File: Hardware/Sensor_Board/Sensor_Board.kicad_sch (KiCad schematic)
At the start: 3 parts, among them J2 Conn_02x20_Odd_Even

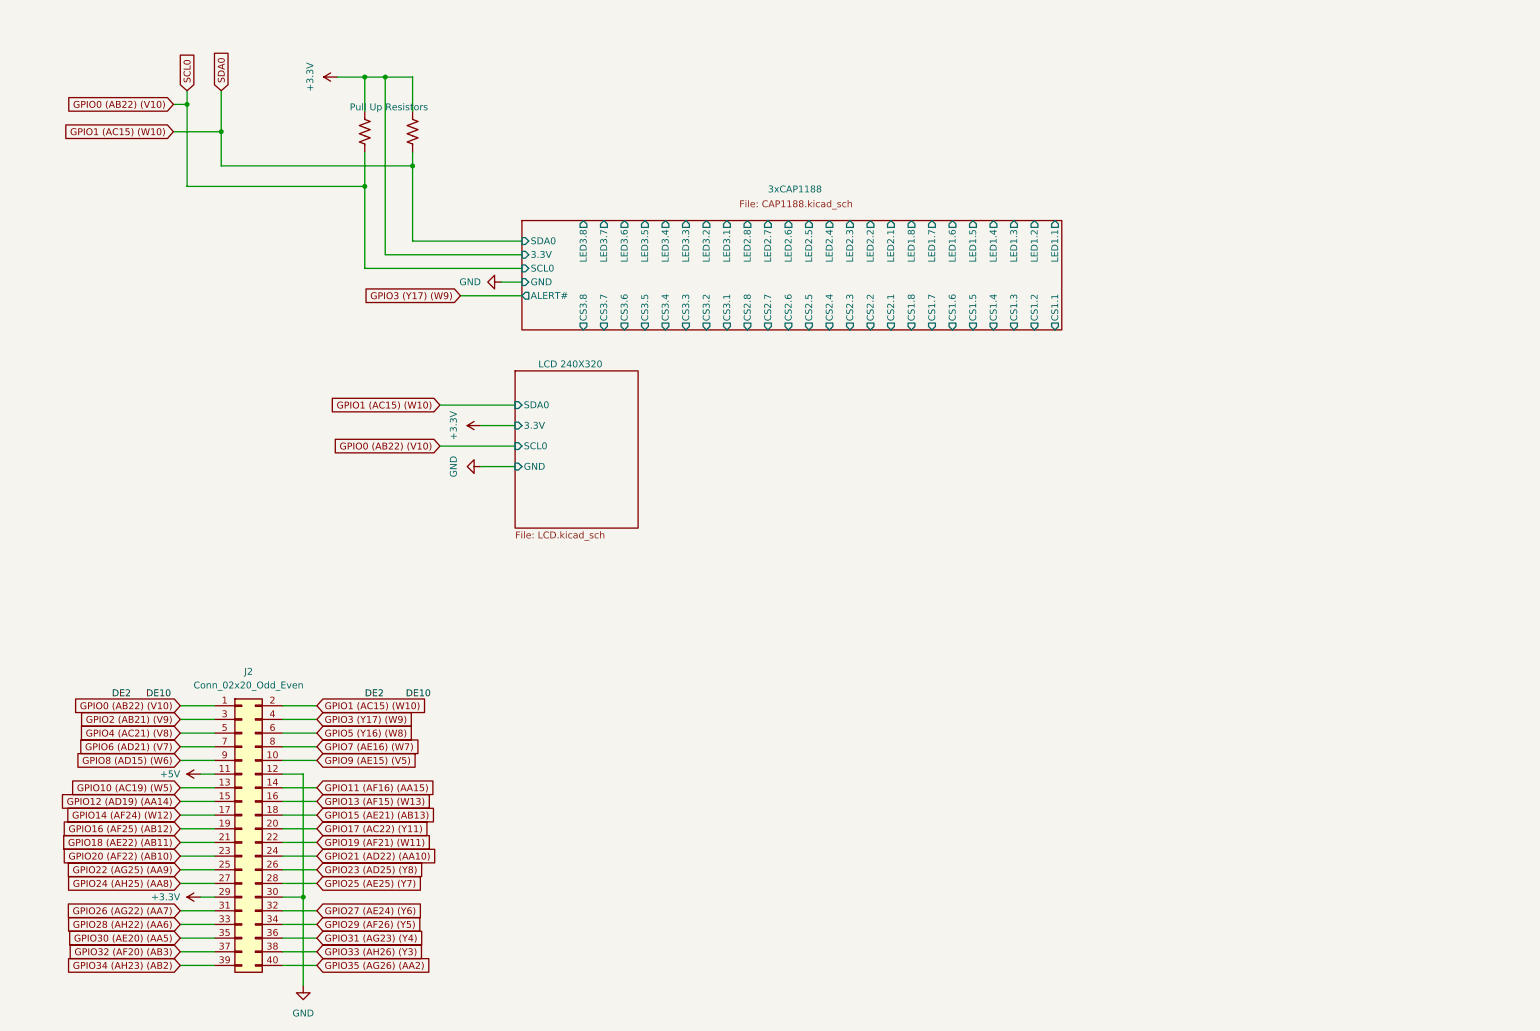
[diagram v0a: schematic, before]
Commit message: Add files via upload
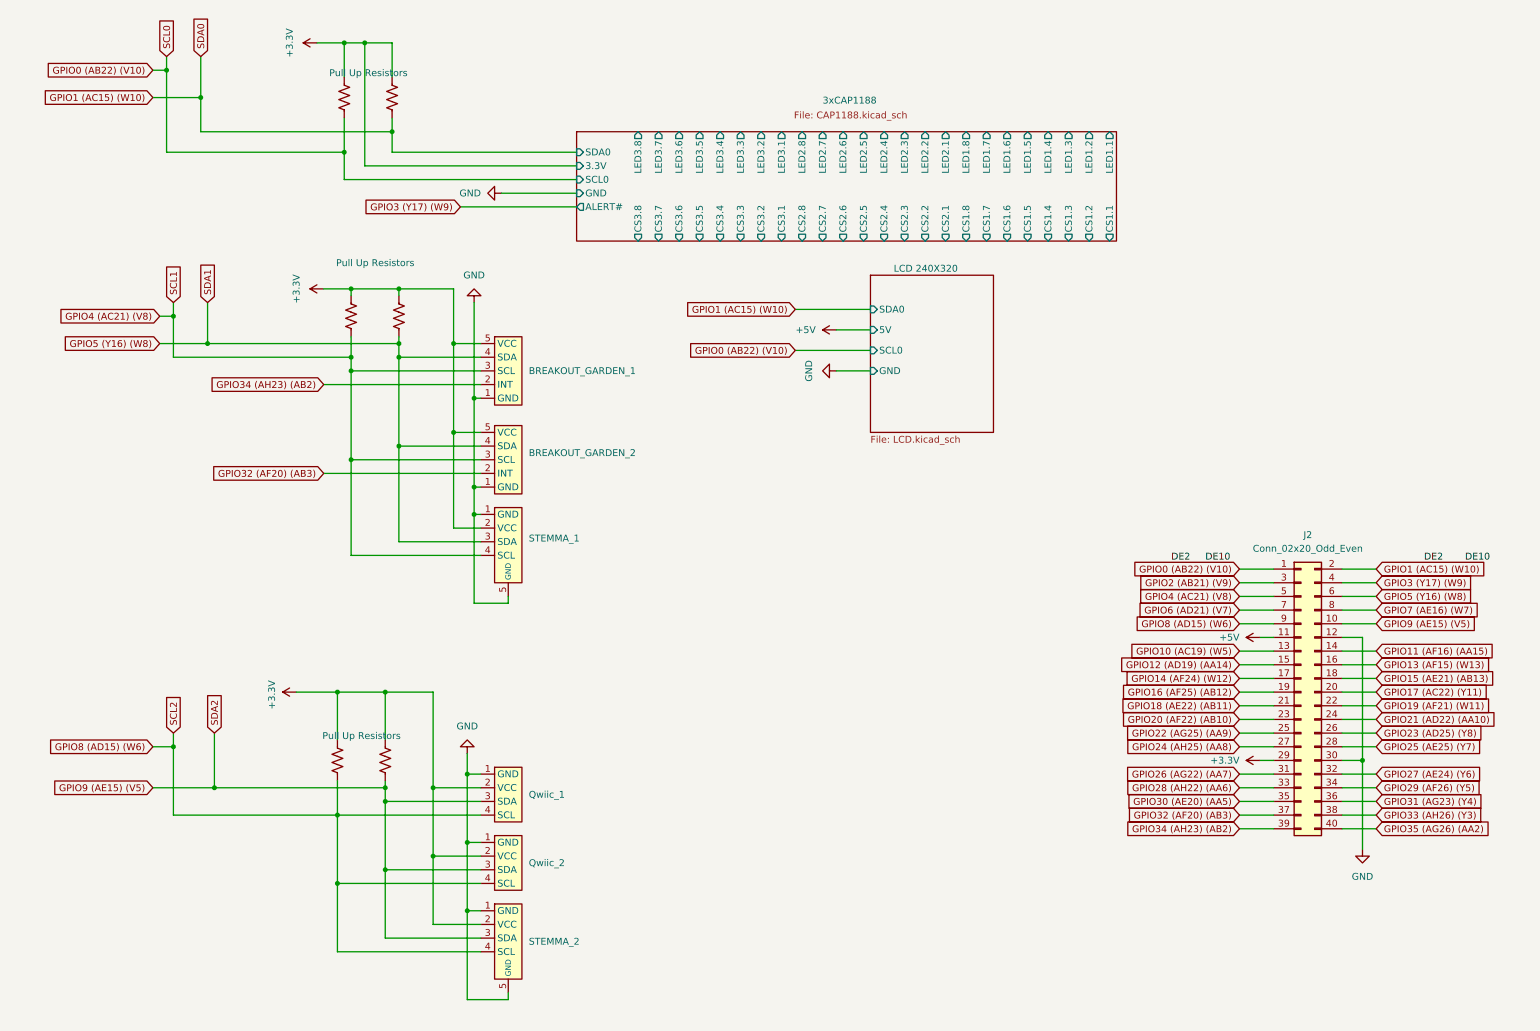
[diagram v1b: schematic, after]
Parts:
- added BREAKOUT_GARDEN_1, BREAKOUT_GARDEN_2: ~, symbol Sensor_Board:BG_I2C
- added Qwiic_1, Qwiic_2: ~, symbol Sensor_Board:Qwiic_Connector
- added R3, R5: Pull Up Resistors, symbol Device:R_US
- added R4, R6: Pull Up Resistor, symbol Device:R_US
- added STEMMA_1, STEMMA_2: ~, symbol Sensor_Board:STEMMA_QT_JST_SH
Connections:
- net +3.3V: now also BREAKOUT_GARDEN_1.5 (VCC), BREAKOUT_GARDEN_2.5 (VCC), Qwiic_1.2 (VCC), Qwiic_2.2 (VCC), R3.1, R4.1, R5.1, R6.1, STEMMA_1.2 (VCC), STEMMA_2.2 (VCC)
- net GND: now also BREAKOUT_GARDEN_1.1 (GND), BREAKOUT_GARDEN_2.1 (GND), Qwiic_1.1 (GND), Qwiic_2.1 (GND), STEMMA_1.1 (GND), STEMMA_1.5 (GND), STEMMA_2.1 (GND), STEMMA_2.5 (GND)
- net GPIO32 (AF20) (AB3): now also BREAKOUT_GARDEN_2.2 (INT)
- net GPIO34 (AH23) (AB2): now also BREAKOUT_GARDEN_1.2 (INT)
- net GPIO4 (AC21) (V8): now also BREAKOUT_GARDEN_1.3 (SCL), BREAKOUT_GARDEN_2.3 (SCL), R3.2, STEMMA_1.4 (SCL)
- net GPIO5 (Y16) (W8): now also BREAKOUT_GARDEN_1.4 (SDA), BREAKOUT_GARDEN_2.4 (SDA), R4.2, STEMMA_1.3 (SDA)
- net GPIO8 (AD15) (W6): now also Qwiic_1.4 (SCL), Qwiic_2.4 (SCL), R5.2, STEMMA_2.4 (SCL)
- net GPIO9 (AE15) (V5): now also Qwiic_1.3 (SDA), Qwiic_2.3 (SDA), R6.2, STEMMA_2.3 (SDA)
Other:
- sheet LCD 240X320 ports: added 5V; removed 3.3V
- moved on the sheet: J2
